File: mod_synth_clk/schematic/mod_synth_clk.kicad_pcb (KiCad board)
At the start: 2 copper layers, 17.8 x 113 mm, 9 parts, among them J1 Clock, J2 Conn_02x08_Odd_Even

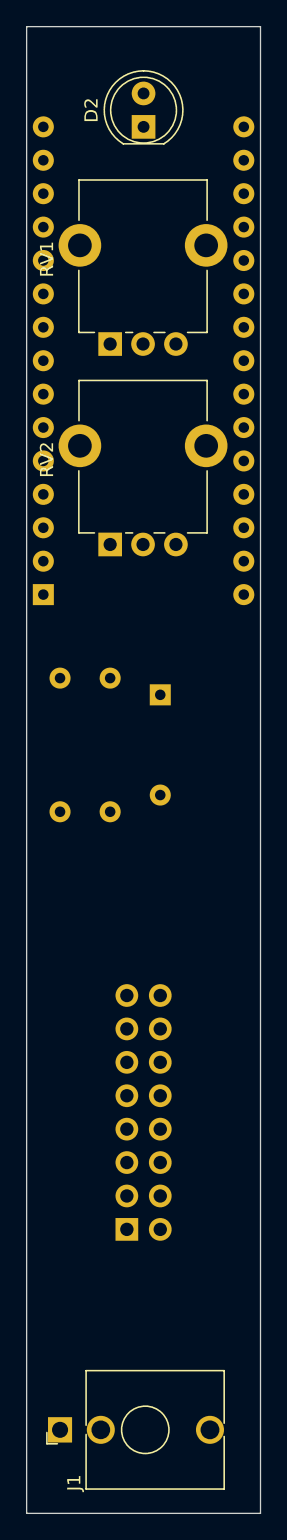
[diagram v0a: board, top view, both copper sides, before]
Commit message: Layout clock board
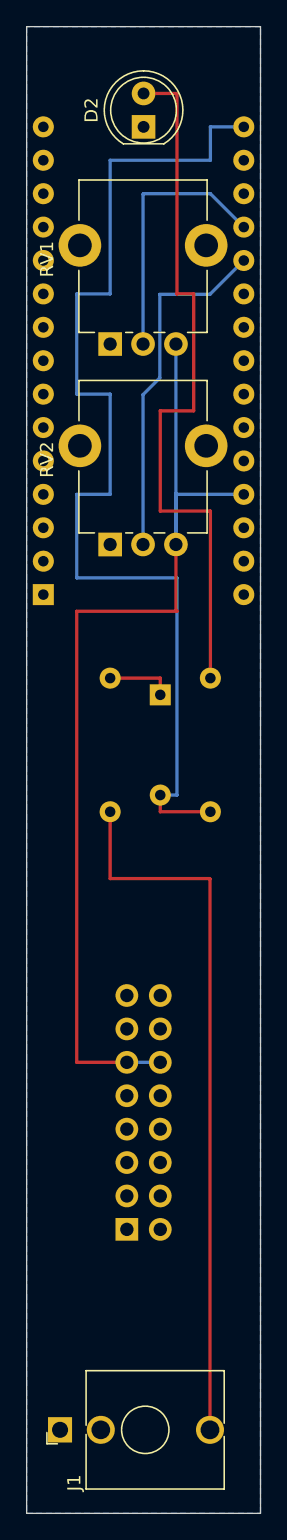
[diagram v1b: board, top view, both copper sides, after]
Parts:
- moved R2 15.3 mm to (52.1, 74.9), turned to 270 degrees
- moved R1 10.2 mm to (44.5, 74.9), turned to 270 degrees
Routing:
- net Net-(A1-Pad16): track 0.00 -> 82.6 mm
- net +5V: track 0.00 -> 77.5 mm
- net Net-(D2-Pad2): track 0.00 -> 54.6 mm
- net Net-(J1-PadT): track 0.00 -> 54.6 mm
- net Net-(A1-Pad20): track 0.00 -> 27.0 mm
- net Net-(A1-Pad19): track 0.00 -> 20.1 mm
- net Net-(D1-Pad1): track 0.00 -> 5.08 mm
- added copper zone on B.Cu, net GND
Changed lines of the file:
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@@
     (thickness 1.6)
     (drawings 4)
-    (tracks 0)
+    (tracks 49)
     (zones 0)
     (modules 9)
@@
   )
   (module Resistor_THT:R_Axial_DIN0207_L6.3mm_D2.5mm_P10.16mm_Horizontal (layer B.Cu)
-    (at 40.64 85.09 90)
+    (at 52.07 74.93 270)
     (descr "Resistor, Axial_DIN0207 series, Axial, Horizontal, pin pitch=10.16mm, 0.25W = 1/4W, length*diameter=6.3*2.5mm^2, http://cdn-reichelt.de/documents/datenblatt/B400/1_4W%23YAG.pdf")
     (tags "Resistor Axial_DIN0207 series Axial Horizontal pin pitch 10.16mm 0.25W = 1/4W length 6.3mm diameter 2.5mm")
-    (fp_text reference R2 (at 5.08 2.37 -90) (layer B.SilkS)
-      (effects (font (size 1 1) (thickness 0.15)) (justify mirror))
-    )
-    (fp_text value 1k (at 5.08 -2.37 -90) (layer B.Fab)
-      (effects (font (size 1 1) (thickness 0.15)) (justify mirror))
-    )
-    (fp_text user %R (at 5.08 0 -90) (layer B.Fab)
+    (fp_text reference R2 (at 5.08 2.37 270) (layer B.SilkS)
+      (effects (font (size 1 1) (thickness 0.15)) (justify mirror))
+    )
+    (fp_text value 1k (at 5.08 -2.37 270) (layer B.Fab)
+      (effects (font (size 1 1) (thickness 0.15)) (justify mirror))
+    )
+    (fp_text user %R (at 5.08 0 270) (layer B.Fab)
       (effects (font (size 1 1) (thickness 0.15)) (justify mirror))
     )
@@
     (fp_line (start 1.93 -1.25) (end 8.23 -1.25) (layer B.Fab) (width 0.1))
     (fp_line (start 1.93 1.25) (end 1.93 -1.25) (layer B.Fab) (width 0.1))
-    (pad 2 thru_hole oval (at 10.16 0 90) (size 1.6 1.6) (drill 0.8) (layers *.Cu *.Mask)
+    (pad 2 thru_hole oval (at 10.16 0 270) (size 1.6 1.6) (drill 0.8) (layers *.Cu *.Mask)
       (net 1 "Net-(A1-Pad16)"))
-    (pad 1 thru_hole circle (at 0 0 90) (size 1.6 1.6) (drill 0.8) (layers *.Cu *.Mask)
+    (pad 1 thru_hole circle (at 0 0 270) (size 1.6 1.6) (drill 0.8) (layers *.Cu *.Mask)
       (net 32 "Net-(D2-Pad2)"))
     (model ${KISYS3DMOD}/Resistor_THT.3dshapes/R_Axial_DIN0207_L6.3mm_D2.5mm_P10.16mm_Horizontal.wrl
@@
   )
   (module Resistor_THT:R_Axial_DIN0207_L6.3mm_D2.5mm_P10.16mm_Horizontal (layer B.Cu)
-    (at 44.45 85.09 90)
+    (at 44.45 74.93 270)
     (descr "Resistor, Axial_DIN0207 series, Axial, Horizontal, pin pitch=10.16mm, 0.25W = 1/4W, length*diameter=6.3*2.5mm^2, http://cdn-reichelt.de/documents/datenblatt/B400/1_4W%23YAG.pdf")
     (tags "Resistor Axial_DIN0207 series Axial Horizontal pin pitch 10.16mm 0.25W = 1/4W length 6.3mm diameter 2.5mm")
-    (fp_text reference R1 (at 5.08 2.37 -90) (layer B.SilkS)
-      (effects (font (size 1 1) (thickness 0.15)) (justify mirror))
-    )
-    (fp_text value 1k (at 5.08 -2.37 -90) (layer B.Fab)
-      (effects (font (size 1 1) (thickness 0.15)) (justify mirror))
-    )
-    (fp_text user %R (at 5.08 0 -90) (layer B.Fab)
+    (fp_text reference R1 (at 5.08 2.37 270) (layer B.SilkS)
+      (effects (font (size 1 1) (thickness 0.15)) (justify mirror))
+    )
+    (fp_text value 1k (at 5.08 -2.37 270) (layer B.Fab)
+      (effects (font (size 1 1) (thickness 0.15)) (justify mirror))
+    )
+    (fp_text user %R (at 5.08 0 270) (layer B.Fab)
       (effects (font (size 1 1) (thickness 0.15)) (justify mirror))
     )
@@
     (fp_line (start 1.93 -1.25) (end 8.23 -1.25) (layer B.Fab) (width 0.1))
     (fp_line (start 1.93 1.25) (end 1.93 -1.25) (layer B.Fab) (width 0.1))
-    (pad 2 thru_hole oval (at 10.16 0 90) (size 1.6 1.6) (drill 0.8) (layers *.Cu *.Mask)
+    (pad 2 thru_hole oval (at 10.16 0 270) (size 1.6 1.6) (drill 0.8) (layers *.Cu *.Mask)
       (net 33 "Net-(J1-PadT)"))
-    (pad 1 thru_hole circle (at 0 0 90) (size 1.6 1.6) (drill 0.8) (layers *.Cu *.Mask)
+    (pad 1 thru_hole circle (at 0 0 270) (size 1.6 1.6) (drill 0.8) (layers *.Cu *.Mask)
       (net 31 "Net-(D1-Pad1)"))
     (model ${KISYS3DMOD}/Resistor_THT.3dshapes/R_Axial_DIN0207_L6.3mm_D2.5mm_P10.16mm_Horizontal.wrl
@@
   (gr_line (start 38.1 138.43) (end 55.88 138.43) (layer Edge.Cuts) (width 0.05))
   (gr_line (start 38.1 25.4) (end 38.1 138.43) (layer Edge.Cuts) (width 0.05))
+  (segment (start 48.26 83.82) (end 48.26 85.09) (width 0.25) (layer F.Cu) (net 1))
+  (segment (start 48.26 85.09) (end 52.07 85.09) (width 0.25) (layer F.Cu) (net 1))
+  (segment (start 44.45 45.72) (end 44.45 35.56) (width 0.25) (layer B.Cu) (net 1))
+  (segment (start 52.07 33.02) (end 54.61 33.02) (width 0.25) (layer B.Cu) (net 1))
+  (segment (start 44.45 35.56) (end 52.07 35.56) (width 0.25) (layer B.Cu) (net 1))
+  (segment (start 41.91 53.34) (end 41.91 45.72) (width 0.25) (layer B.Cu) (net 1))
+  (segment (start 52.07 35.56) (end 52.07 33.02) (width 0.25) (layer B.Cu) (net 1))
+  (segment (start 49.53 83.82) (end 49.53 67.31) (width 0.25) (layer B.Cu) (net 1))
+  (segment (start 44.45 53.34) (end 41.91 53.34) (width 0.25) (layer B.Cu) (net 1))
+  (segment (start 48.26 83.82) (end 49.53 83.82) (width 0.25) (layer B.Cu) (net 1))
+  (segment (start 49.53 67.31) (end 41.91 67.31) (width 0.25) (layer B.Cu) (net 1))
+  (segment (start 41.91 67.31) (end 41.91 60.96) (width 0.25) (layer B.Cu) (net 1))
+  (segment (start 41.91 45.72) (end 44.45 45.72) (width 0.25) (layer B.Cu) (net 1))
+  (segment (start 41.91 60.96) (end 44.45 60.96) (width 0.25) (layer B.Cu) (net 1))
+  (segment (start 44.45 60.96) (end 44.45 53.34) (width 0.25) (layer B.Cu) (net 1))
+  (segment (start 45.72 104.14) (end 48.26 104.14) (width 0.25) (layer B.Cu) (net 9))
+  (segment (start 45.72 104.14) (end 41.91 104.14) (width 0.25) (layer F.Cu) (net 9))
+  (segment (start 41.91 104.14) (end 41.91 69.85) (width 0.25) (layer F.Cu) (net 9))
+  (segment (start 41.91 69.85) (end 49.53 69.85) (width 0.25) (layer F.Cu) (net 9))
+  (segment (start 49.45 69.77) (end 49.45 64.77) (width 0.25) (layer F.Cu) (net 9))
+  (segment (start 49.53 69.85) (end 49.45 69.77) (width 0.25) (layer F.Cu) (net 9))
+  (segment (start 54.61 60.96) (end 49.53 60.96) (width 0.25) (layer B.Cu) (net 9))
+  (segment (start 49.45 61.04) (end 49.45 64.77) (width 0.25) (layer B.Cu) (net 9))
+  (segment (start 49.53 60.96) (end 49.45 61.04) (width 0.25) (layer B.Cu) (net 9))
+  (segment (start 49.45 49.53) (end 49.45 60.88) (width 0.25) (layer B.Cu) (net 9))
+  (segment (start 49.45 60.88) (end 49.45 64.77) (width 0.25) (layer B.Cu) (net 9))
+  (segment (start 52.034999 45.755001) (end 54.61 43.18) (width 0.25) (layer B.Cu) (net 23))
+  (segment (start 48.224999 45.755001) (end 52.034999 45.755001) (width 0.25) (layer B.Cu) (net 23))
+  (segment (start 48.224999 52.105001) (end 48.224999 45.755001) (width 0.25) (layer B.Cu) (net 23))
+  (segment (start 46.95 64.77) (end 46.95 53.38) (width 0.25) (layer B.Cu) (net 23))
+  (segment (start 46.95 53.38) (end 48.224999 52.105001) (width 0.25) (layer B.Cu) (net 23))
+  (segment (start 54.61 40.64) (end 52.07 38.1) (width 0.25) (layer B.Cu) (net 25))
+  (segment (start 52.07 38.1) (end 46.99 38.1) (width 0.25) (layer B.Cu) (net 25))
+  (segment (start 46.95 38.14) (end 46.95 49.53) (width 0.25) (layer B.Cu) (net 25))
+  (segment (start 46.99 38.1) (end 46.95 38.14) (width 0.25) (layer B.Cu) (net 25))
+  (segment (start 44.45 74.93) (end 48.26 74.93) (width 0.25) (layer F.Cu) (net 31))
+  (segment (start 48.26 74.93) (end 48.26 76.2) (width 0.25) (layer F.Cu) (net 31))
+  (segment (start 52.07 62.23) (end 52.07 74.93) (width 0.25) (layer F.Cu) (net 32))
+  (segment (start 48.26 62.23) (end 52.07 62.23) (width 0.25) (layer F.Cu) (net 32))
+  (segment (start 49.53 30.48) (end 49.53 45.72) (width 0.25) (layer F.Cu) (net 32))
+  (segment (start 49.53 45.72) (end 50.8 45.72) (width 0.25) (layer F.Cu) (net 32))
+  (segment (start 50.8 45.72) (end 50.8 54.61) (width 0.25) (layer F.Cu) (net 32))
+  (segment (start 46.99 30.48) (end 49.53 30.48) (width 0.25) (layer F.Cu) (net 32))
+  (segment (start 50.8 54.61) (end 48.26 54.61) (width 0.25) (layer F.Cu) (net 32))
+  (segment (start 48.26 54.61) (end 48.26 62.23) (width 0.25) (layer F.Cu) (net 32))
+  (segment (start 52.04 132.08) (end 52.04 90.2) (width 0.25) (layer F.Cu) (net 33))
+  (segment (start 52.04 90.2) (end 52.01 90.17) (width 0.25) (layer F.Cu) (net 33))
+  (segment (start 52.01 90.17) (end 44.45 90.17) (width 0.25) (layer F.Cu) (net 33))
+  (segment (start 44.45 90.17) (end 44.45 85.09) (width 0.25) (layer F.Cu) (net 33))
+  (zone (net 5) (net_name GND) (layer B.Cu) (hatch edge 0.508)
+    (connect_pads (clearance 0.508))
+    (min_thickness 0.254)
+    (fill yes (arc_segments 32) (thermal_gap 0.508) (thermal_bridge_width 0.508))
+    (polygon
+      (pts
+        (xy 38.1 138.43) (xy 55.88 138.43) (xy 55.88 25.4) (xy 38.1 25.4)
+      )
+    )
+  )
 )
